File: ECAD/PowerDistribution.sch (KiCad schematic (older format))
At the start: 10 parts, among them U60 CD74HC4067SM, U61 CD74HC4067SM, U62 74HC595, U63 74HC595

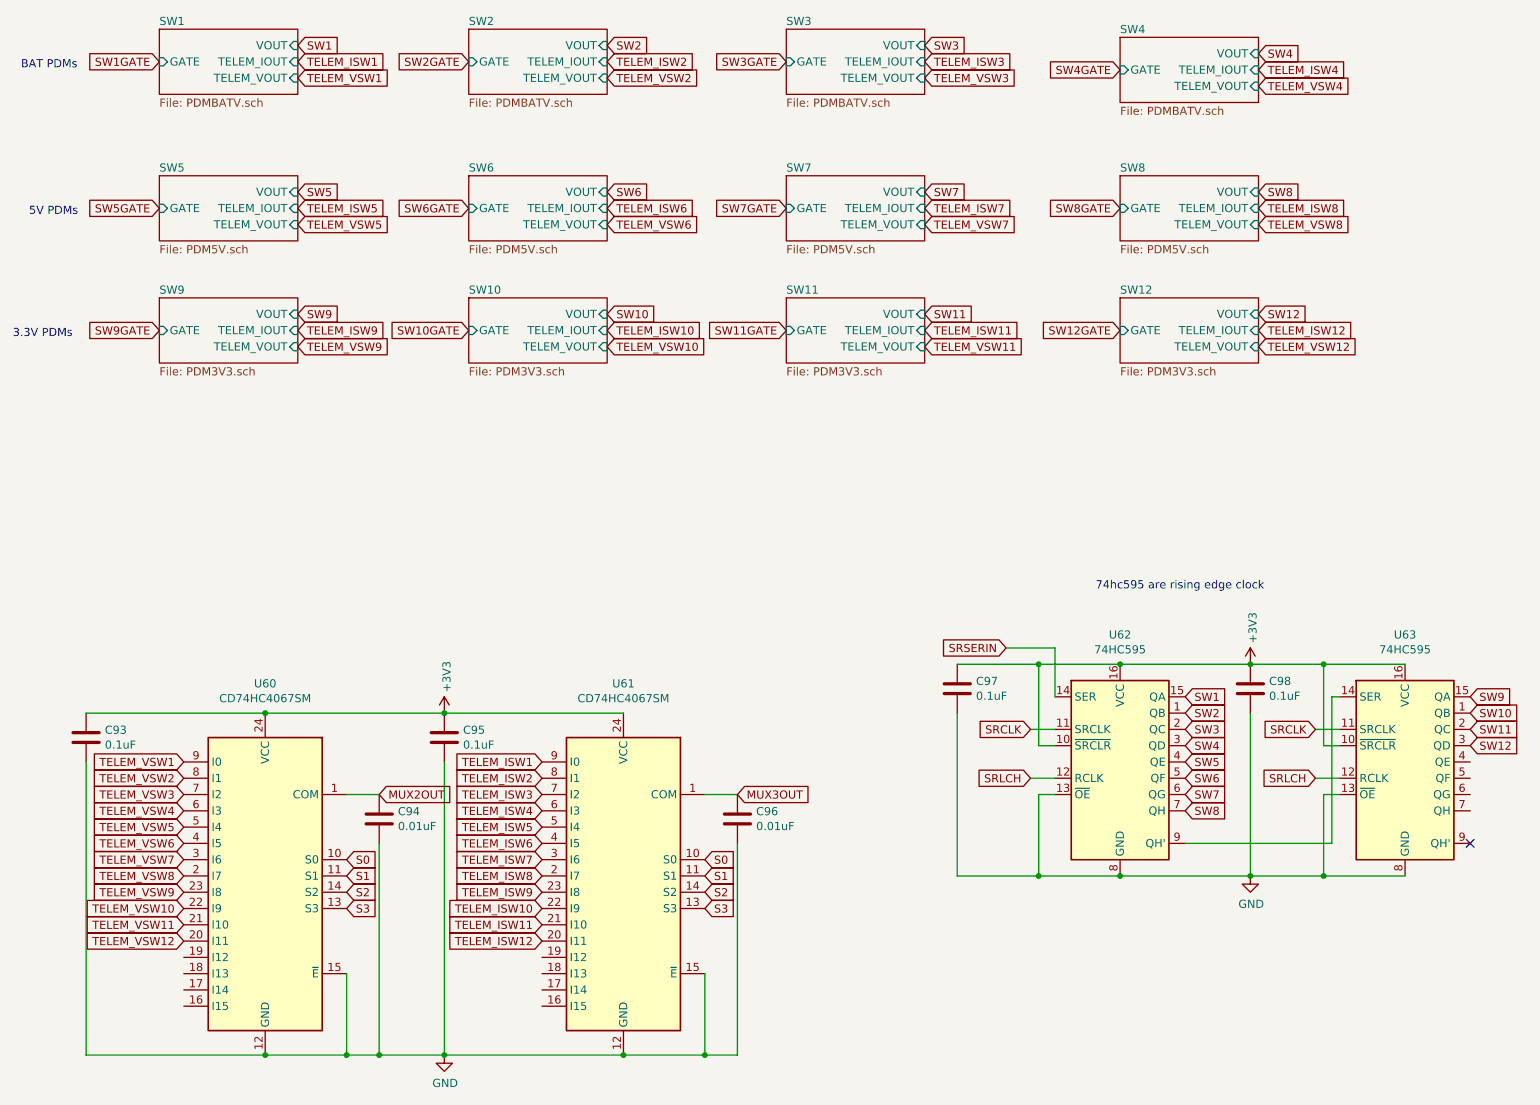
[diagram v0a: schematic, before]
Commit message: Condense muxes and add srrst
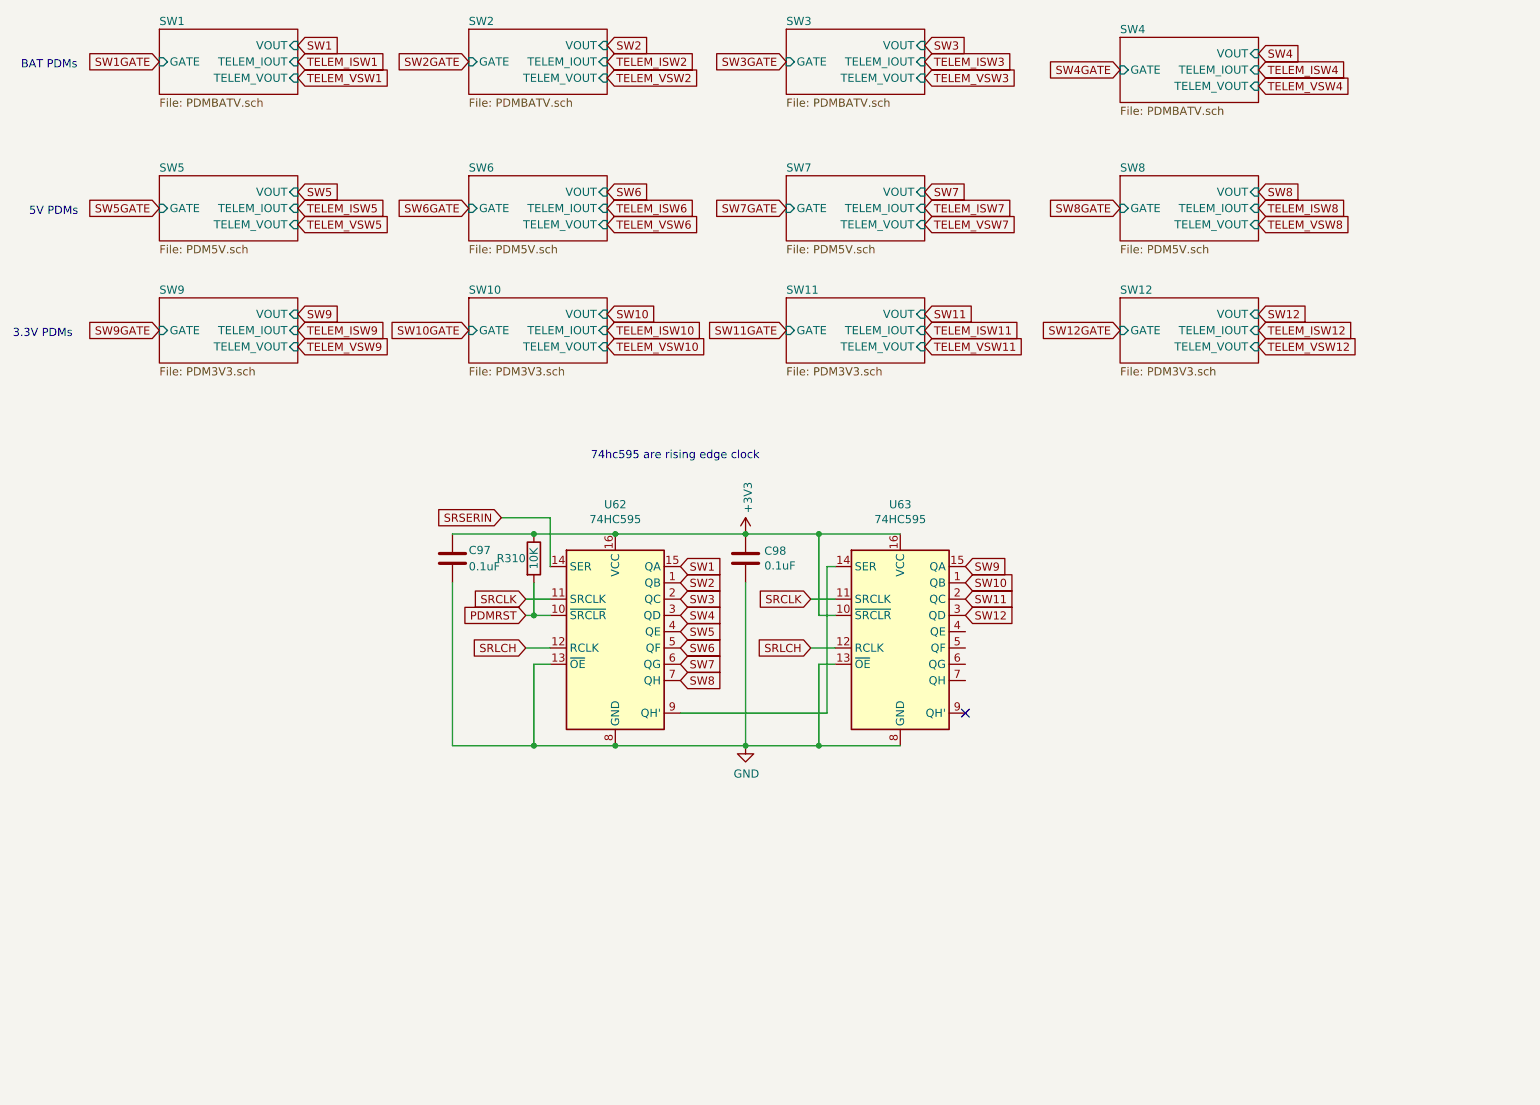
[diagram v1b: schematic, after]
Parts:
- removed C93, C95: 0.1uF, Capacitor_SMD:C_0805_2012Metric, symbol Device:C
- removed C94, C96: 0.01uF, Capacitor_SMD:C_0805_2012Metric, symbol Device:C
- removed U60, U61: CD74HC4067SM, Package_SO:SSOP-24_5.3x8.2mm_P0.65mm, symbol 74xx:CD74HC4067SM
- added R310: 10K, symbol Device:R
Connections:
- net +3V3: now also R310.1; no longer U62.10 (~SRCLR)
- new net PDMRST: R310.2, U62.10 (~SRCLR)
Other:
- moved on the sheet: C97, C98, U62, U63
